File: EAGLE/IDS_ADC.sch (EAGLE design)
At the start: 17 parts, among them IC1 NE5532N, IC2 NE5532N

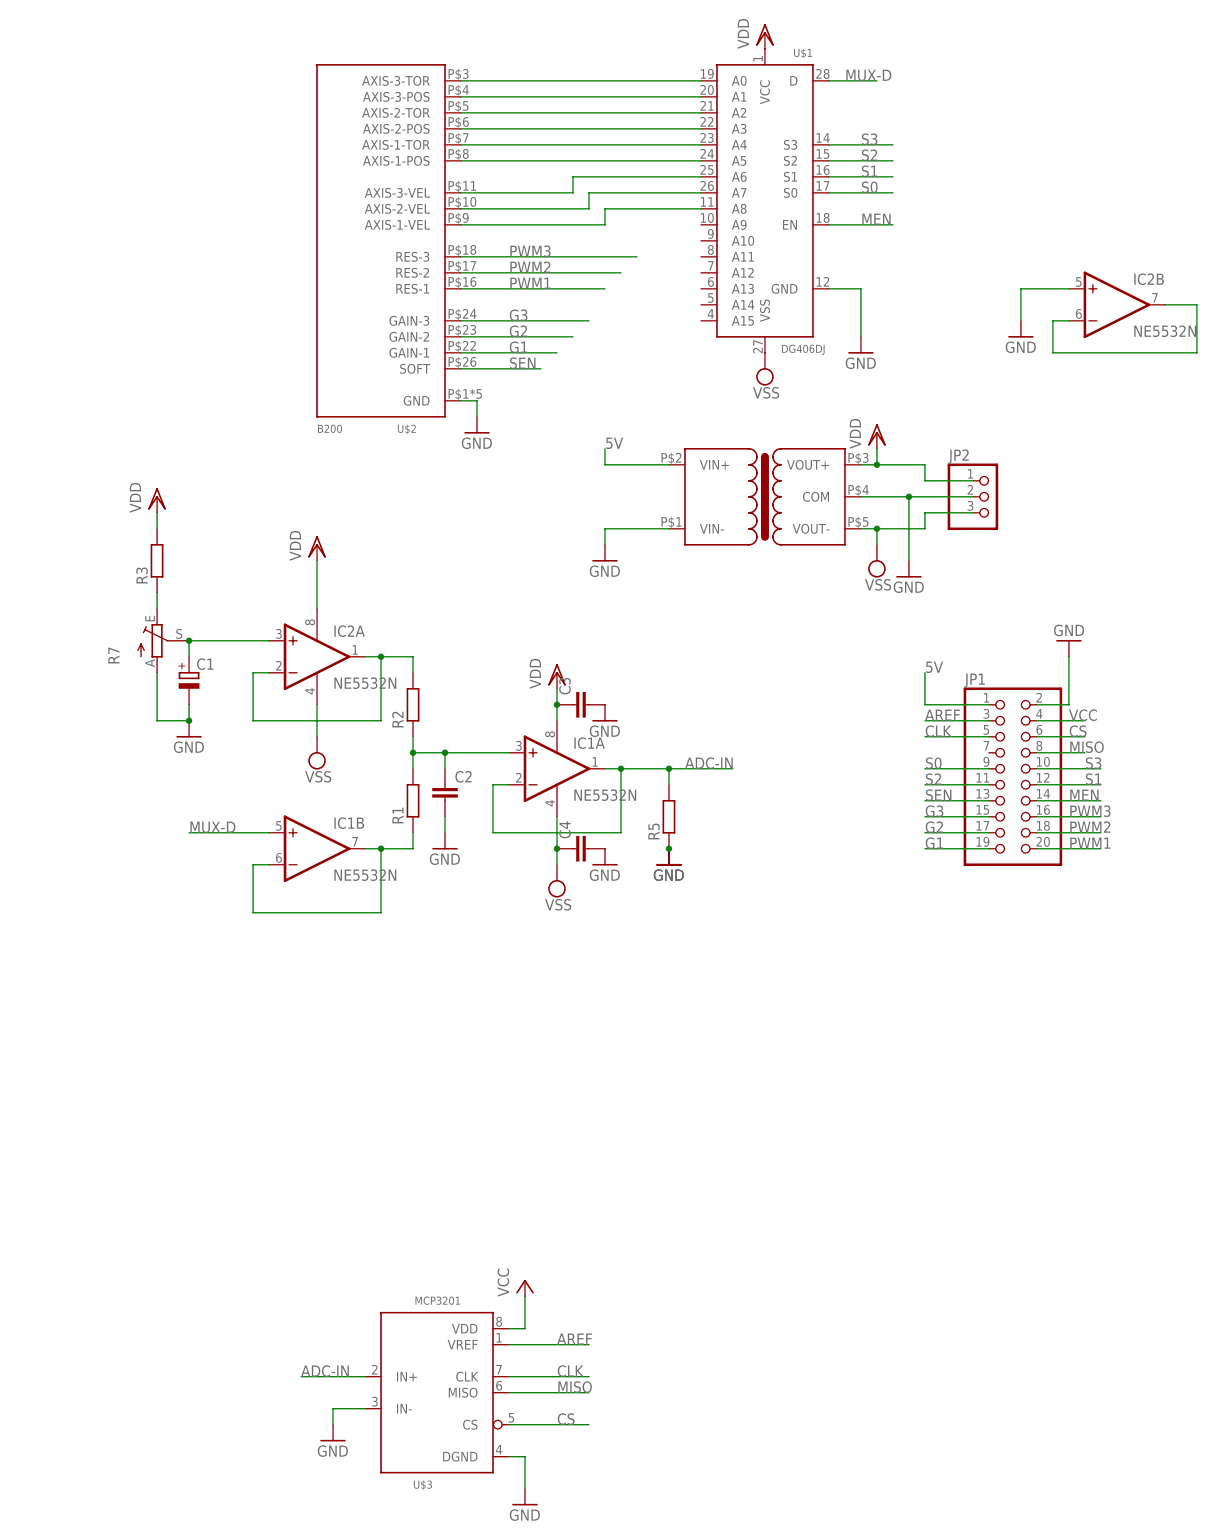
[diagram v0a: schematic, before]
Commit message: Add files via upload
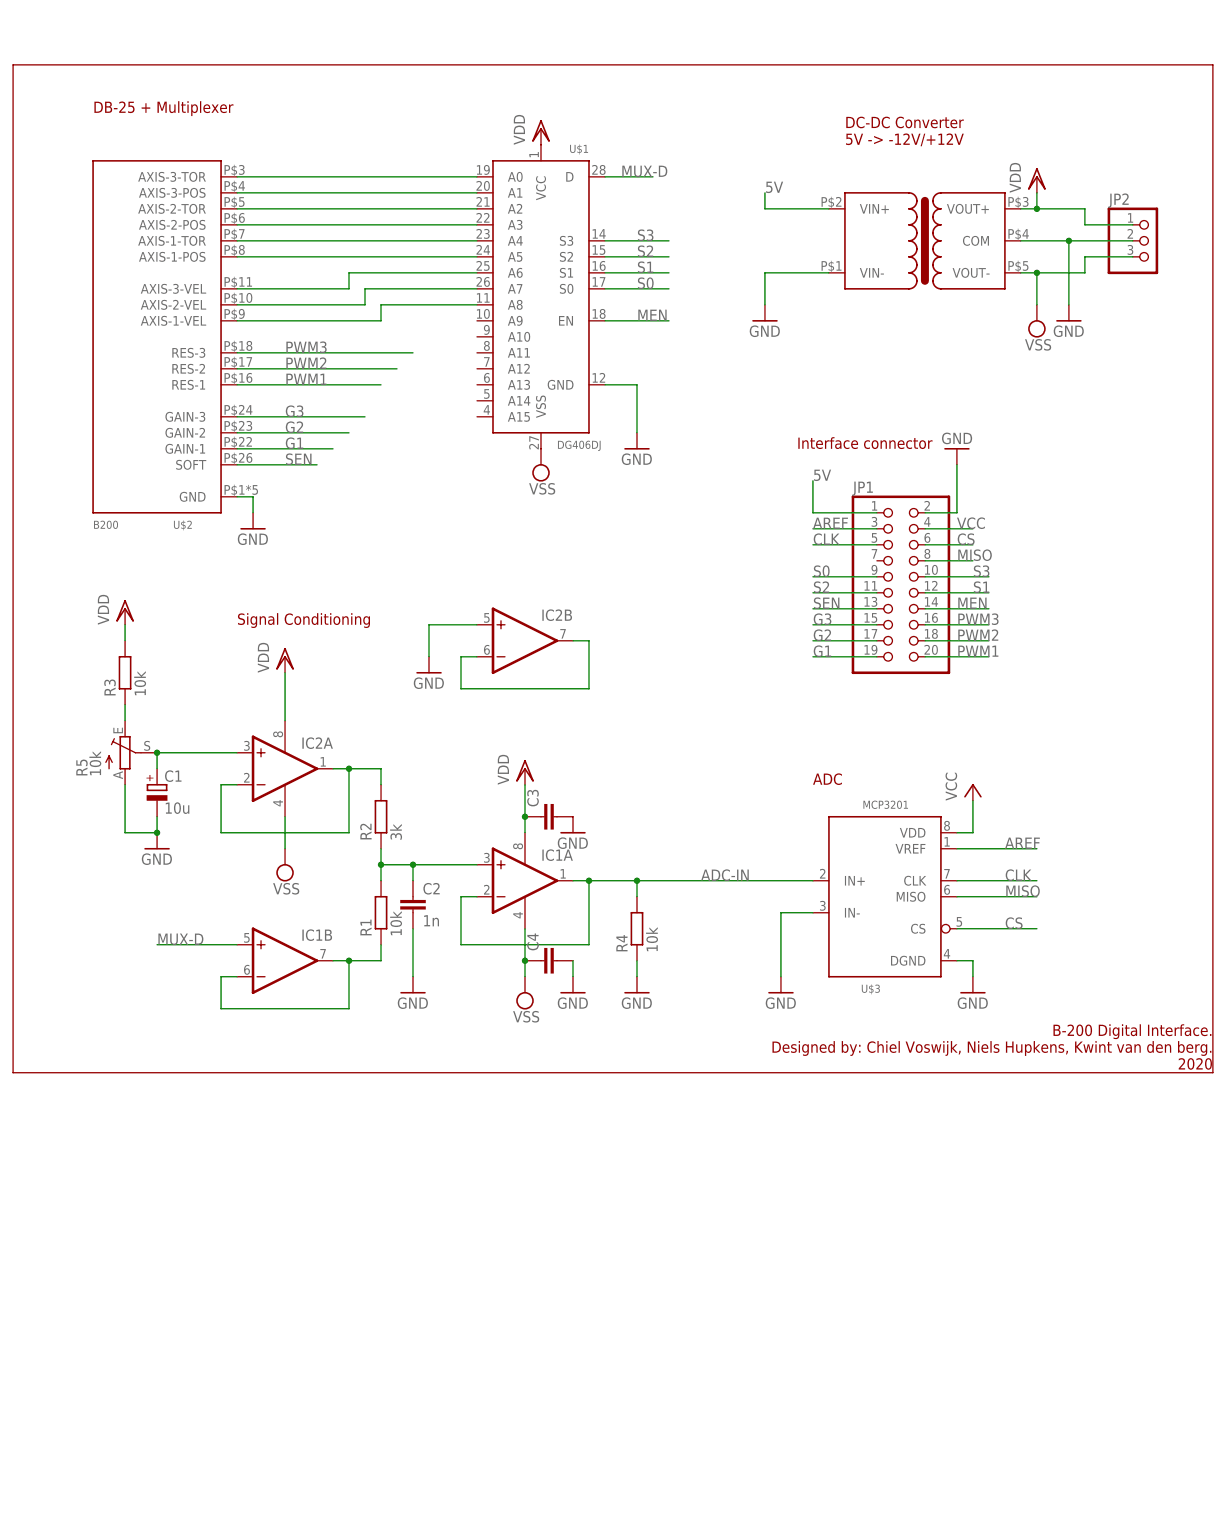
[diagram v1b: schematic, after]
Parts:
- removed R7: (no value), pot:TRIM_EU-RJ9W
- added R4: 10k, rcl:R-EU_0207/7
- C1: value (none) -> 10u; device rcl:CPOL-EUE5-8.5 -> rcl:CPOL-EUE2.5-7
- C2: value (none) -> 1n
- R1, R3: value (none) -> 10k
- R2: value (none) -> 3k
- R5: value (none) -> 10k; device rcl:R-EU_0207/7 -> pot:TRIM_EU-RJ9W
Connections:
- net ADC-IN: now also R4.2; no longer R5.2
- net GND: now also R4.1, R5.A; no longer R5.1, R7.A
- net N$15: now also R5.E; no longer R7.E
- net N$8: now also R5.S; no longer R7.S
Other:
- note added: "ADC"
- note added: "B-200 Digital Interface. Designed by: Chiel Voswijk, Niels Hupkens, Kwint van den berg. 2020"
- note added: "DB-25 + Multiplexer"
- note added: "DC-DC Converter 5V -> -12V/+12V"
- note added: "Interface connector"
- note added: "Signal Conditioning"
- moved on the sheet: C1, C2, C3, C4, IC1A, IC1B, IC2A, IC2B, JP1, JP2, R1, R2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
